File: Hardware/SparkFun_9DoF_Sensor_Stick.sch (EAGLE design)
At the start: 27 parts, among them U1 ITG-32001:1, U2 ADXL345, U4 3.3V

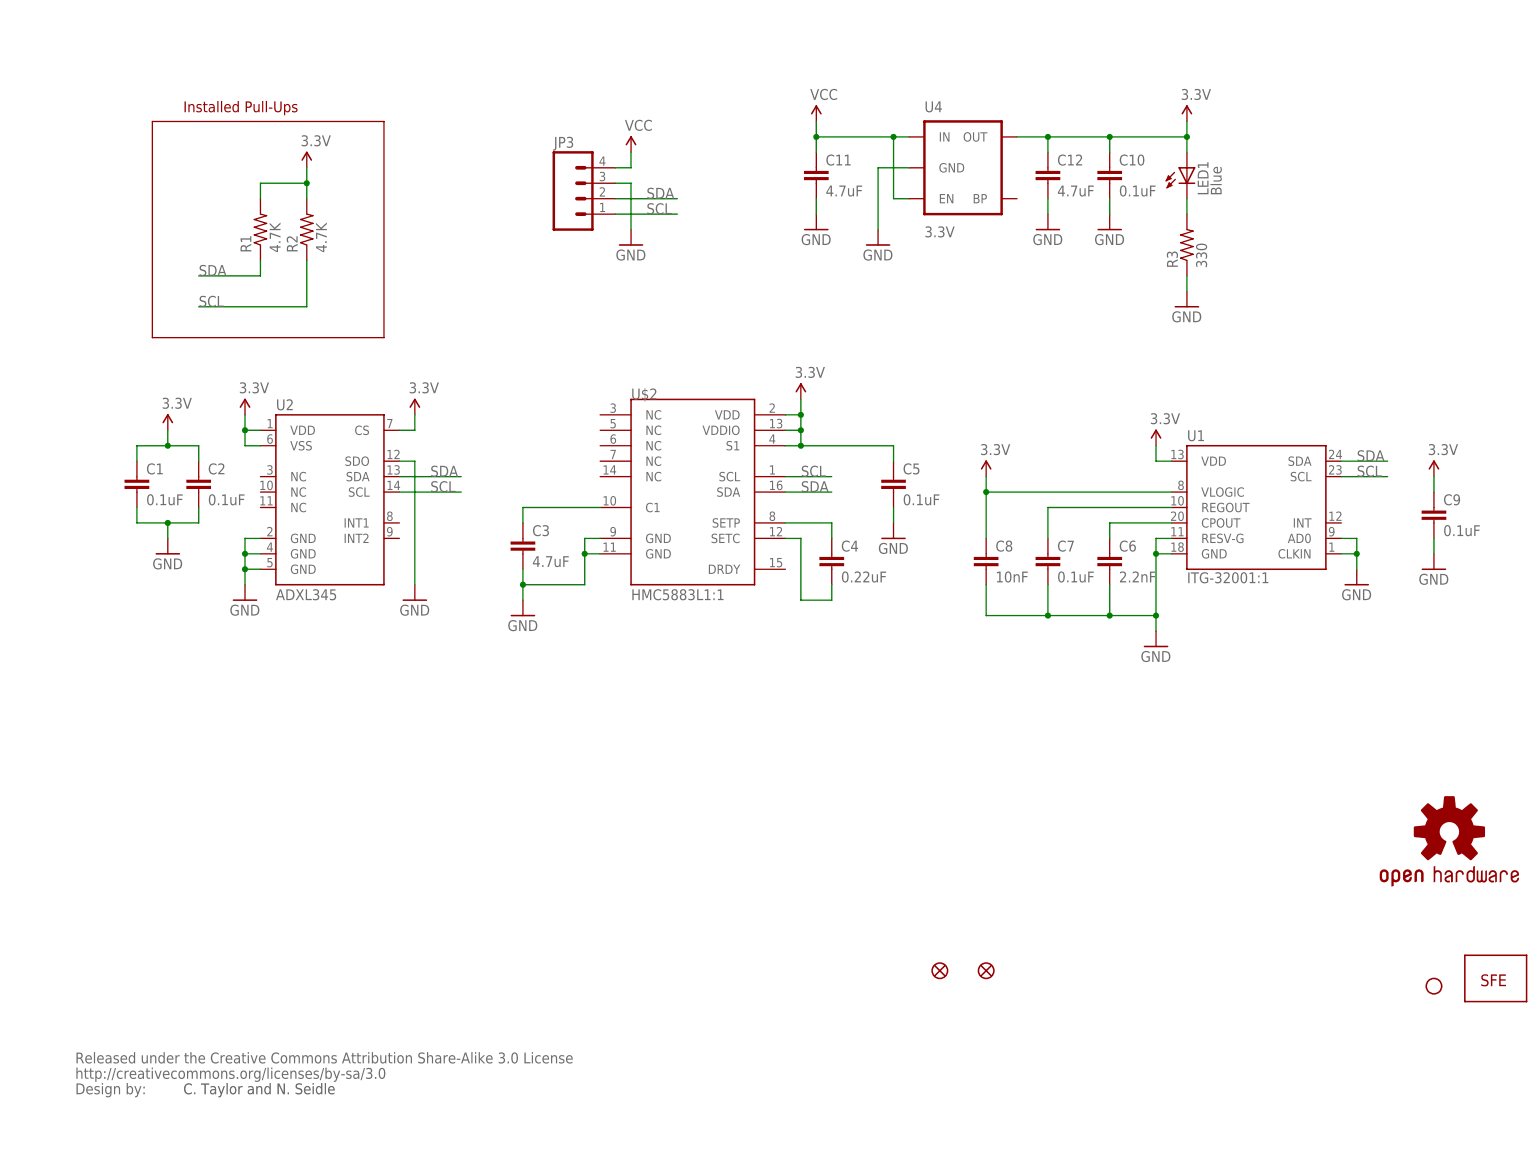
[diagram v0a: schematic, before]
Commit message: Mid revision work - NOT FUNCTIONAL
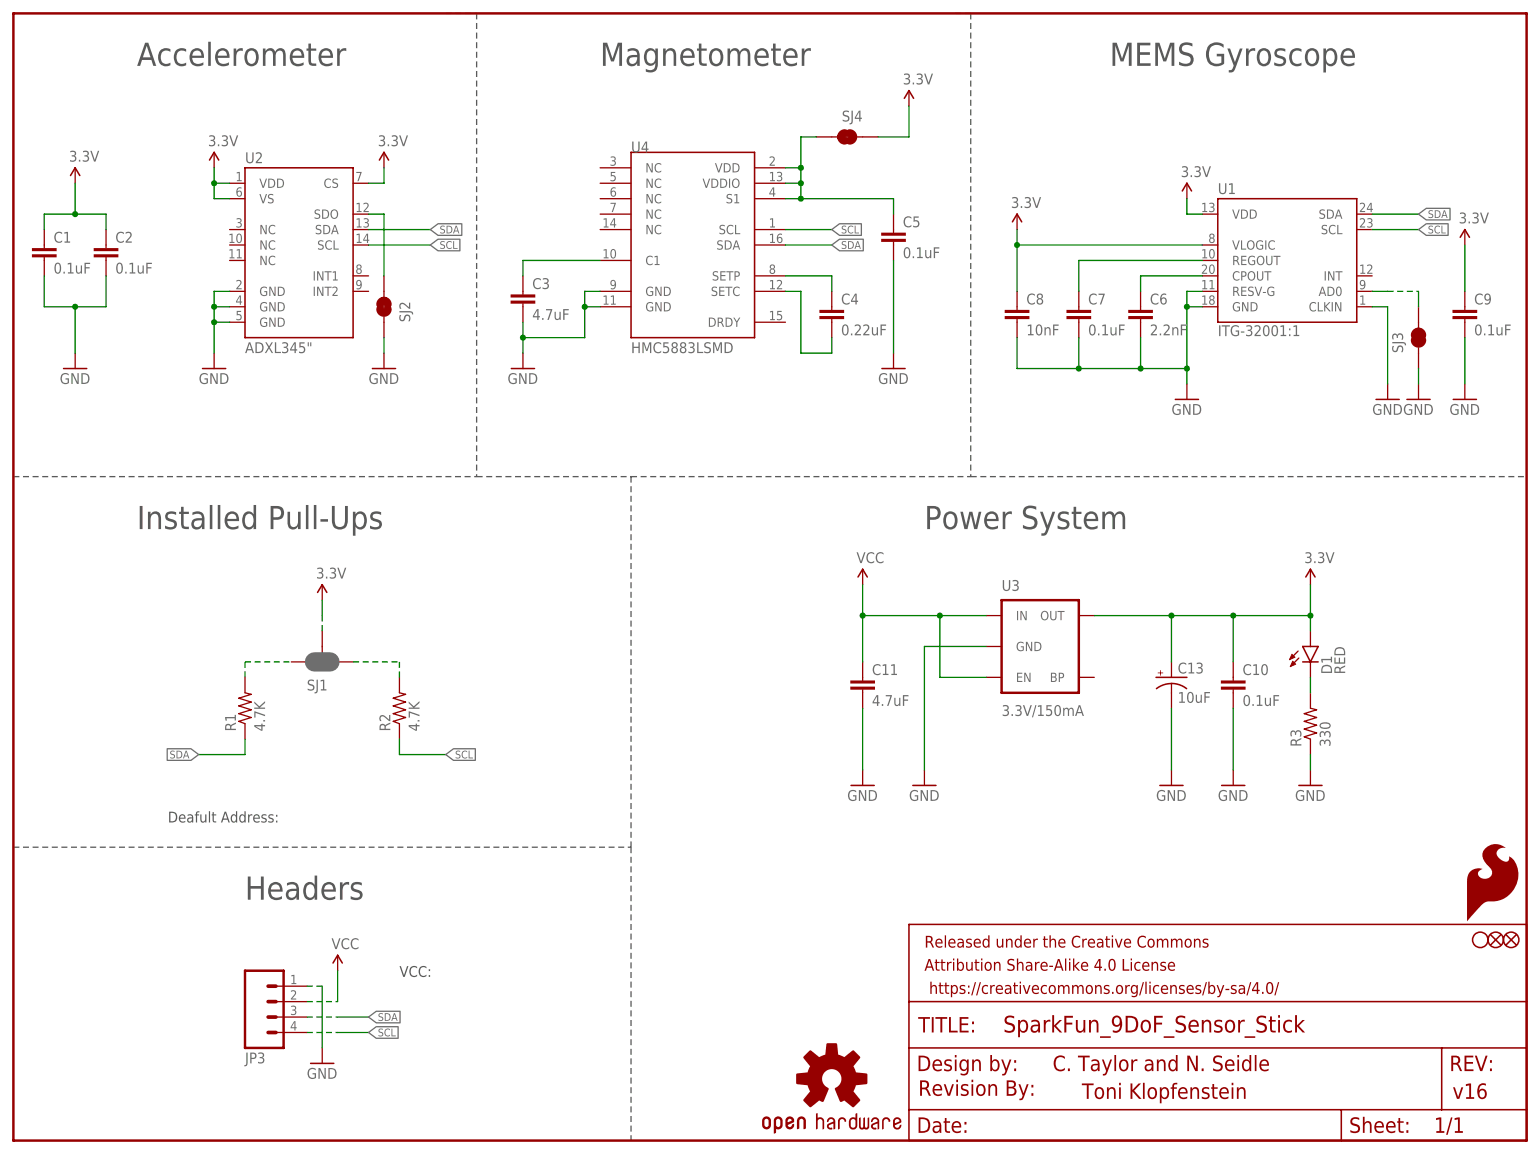
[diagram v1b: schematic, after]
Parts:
- removed C12: 4.7uF, SparkFun:CAP0402-CAP
- removed LED1: Blue, SparkFun:LED0603
- removed U$1: CREATIVE_COMMONS, SparkFun:CREATIVE_COMMONS
- removed U$2: HMC5883L1:1, Testing:HMC5883L1:1
- added C13: 10uF, SparkFun-Capacitors:10UF-16V-10%(TANT)
- added D1: RED, SparkFun-LED:LED-RED0603
- added FRAME1: (no value), SparkFun-Aesthetics:FRAME-LETTER
- added SJ1: JUMPER-PAD-3-NC_BY_PASTE, SparkFun-Passives:JUMPER-PAD-3-NC_BY_PASTE
- added SJ2, SJ3, SJ4: JUMPER-PAD-2-NC_BY_TRACE, SparkFun-Passives:JUMPER-PAD-2-NC_BY_TRACE
- added U$4: REVISION, SparkFun-Aesthetics:REVISION
- added U3: 3.3V/150mA, SparkFun-PowerIC:V_REG_MIC52053.3V
- C1, C10, C2, C5, C7, C9: device SparkFun:CAP0402-CAP -> SparkFun-Capacitors:0.1UF-25V(+80/-20%)(0603)
- C11, C3: device SparkFun:CAP0402-CAP -> SparkFun-Capacitors:4.7UF-6.3V-10%(0603)0603
- C4: device SparkFun:CAP0402-CAP -> SparkFun-Capacitors:0.22UF-25V-10%(0603)
- C6: device SparkFun:CAP0402-CAP -> SparkFun-Capacitors:2.2NF/2200PF-50V-10%(0603)
- C8: device SparkFun:CAP0402-CAP -> SparkFun-Capacitors:10NF/10000PF-50V-10%(0603)
- JP1, JP2: device SparkFun:FIDUCIAL1X2 -> SparkFun-Aesthetics:FIDUCIAL1X2
- JP3: device SparkFun:M04PTH -> SparkFun-Connectors:M04PTH
- JP4: value LOGO-SFESK -> SFE_LOGO_FLAME.1_INCH; device SparkFun:LOGO-SFESK -> SparkFun-Aesthetics:SFE_LOGO_FLAME.1_INCH
- JP5: device SparkFun:STAND-OFF -> SparkFun-Electromechanical:STAND-OFF
- R1, R2: device SparkFun:RESISTOR0402-RES -> SparkFun-Resistors:4.7KOHM-1/10W-1%(0603)
- R3: device SparkFun:RESISTOR0402-RES -> SparkFun-Resistors:330OHM1/10W1%(0603)
- U$3: device SparkFun:OSHW-LOGOS -> SparkFun-Aesthetics:OSHW-LOGOS
- U1: device Testing:ITG-32001:1 -> SparkFun-Sensors:ITG-32001:1
- U2: value ADXL345 -> ADXL345"; device SparkFun:ADXL345 -> SparkFun-Sensors:ADXL345"
- U4: value 3.3V -> HMC5883LSMD; device SparkFun:V_REG_LDOSMD -> SparkFun-Sensors:HMC5883LSMD
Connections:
- new net N$10: SJ2.2, U2.SDO
- new net N$12: C5.1, SJ4.2, U4.S1, U4.VDD, U4.VDDIO
- new net N$6: R1.2, SJ1.3
- new net N$8: R2.2, SJ1.1
- new net N$9: SJ3.2, U1.AD0
- net 3.3V: now also C13.+, D1.A, SJ1.2, SJ4.1, U2.VS, U3.OUT; no longer C12.1, C5.1, LED1.A, R1.2, R2.2, U$2.S1, U$2.VDD, U$2.VDDIO, U2.VSS, U4.OUT
- net GND: now also C13.-, JP3.1, SJ2.1, SJ3.1, U3.GND, U4.GND@1, U4.GND@2; no longer C12.2, JP3.3, U$2.GND@1, U$2.GND@2, U1.AD0, U2.SDO, U4.GND
- net N$1: now also U4.C1; no longer U$2.C1
- net N$2: now also U4.SETP; no longer U$2.SETP
- net N$3: now also U4.SETC; no longer U$2.SETC
- net N$4: now also D1.C; no longer LED1.C
- net SCL: now also JP3.4, U4.SCL; no longer JP3.1, U$2.SCL
- net SDA: now also JP3.3, U4.SDA; no longer JP3.2, U$2.SDA
- net VCC: now also JP3.2, U3.EN, U3.IN; no longer JP3.4, U4.EN, U4.IN
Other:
- note added: "Accelerometer"
- note added: "Deafult Address:"
- note added: "Headers"
- note added: "MEMS Gyroscope"
- note added: "Magnetometer"
- note added: "Power System"
- note added: "Toni Klopfenstein"
- note added: "VCC:"
- note added: "v16"
- moved on the sheet: C1, C10, C11, C2, C3, C4, C5, C6, C7, C8, C9, JP3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
